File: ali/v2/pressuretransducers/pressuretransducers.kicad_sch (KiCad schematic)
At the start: 4 parts

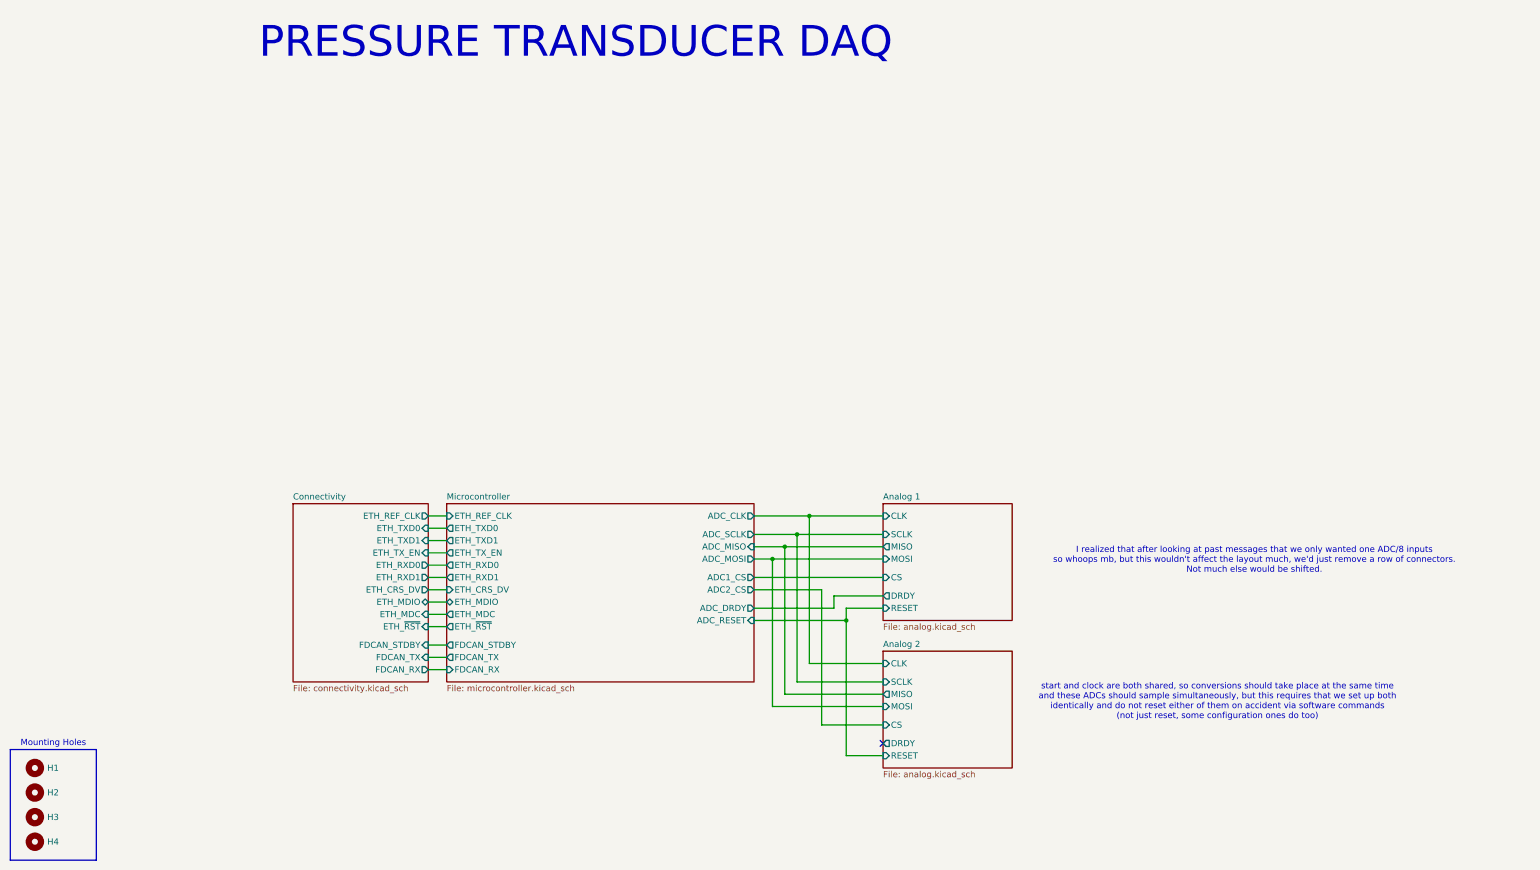
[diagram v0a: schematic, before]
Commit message: Begin prep for second board review
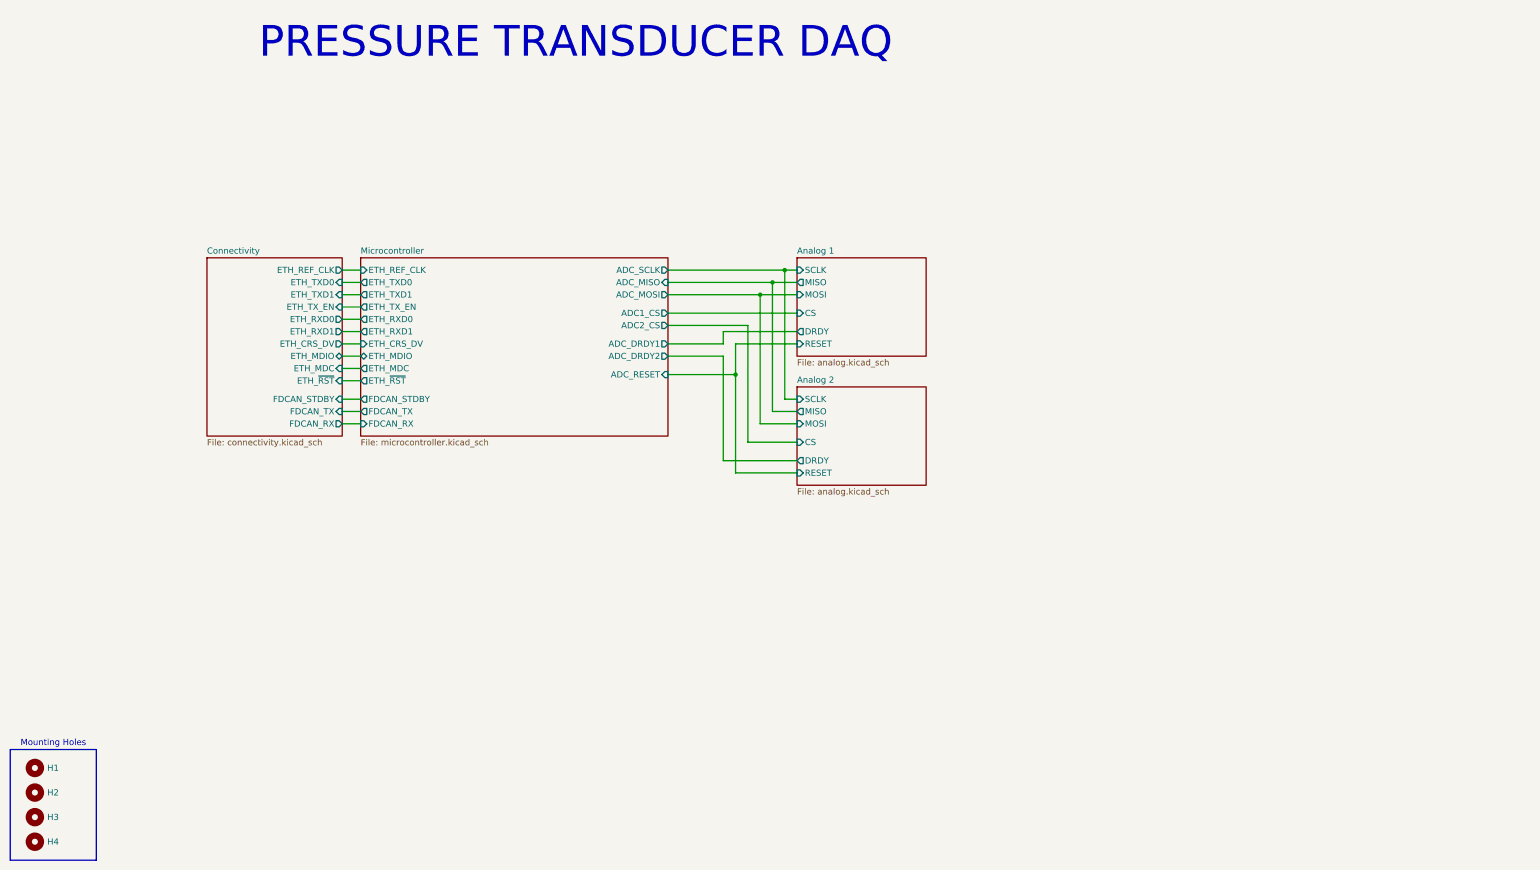
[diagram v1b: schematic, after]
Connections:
- no-connect marks 1 -> 0
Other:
- sheet Analog 1 ports: added none; removed CLK
- sheet Analog 2 ports: added none; removed CLK
- sheet Microcontroller ports: added ADC_DRDY1, ADC_DRDY2; removed ADC_CLK, ADC_DRDY
- note removed: "I realized that after looking at past messages that we only wanted one ADC/8 inputs so whoops mb, but this wouldn't affect the layout much, we'd just remove a row of connectors. Not much else would be shifted."
- note removed: "start and clock are both shared, so conversions should take place at the same time and these ADCs should sample simultaneously, but this requires that we set up both identically and do not reset either of them on accident via software commands (not just reset, some configuration ones do too)"
